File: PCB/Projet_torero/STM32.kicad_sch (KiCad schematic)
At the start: 35 parts, among them J201 Conn_02x07_Odd_Even, J202 Conn_02x08_Odd_Even, SW201 SW_Push, SW202 SW_Push, U201 STM32G431CBUx, Y201 Crystal_GND24_Small

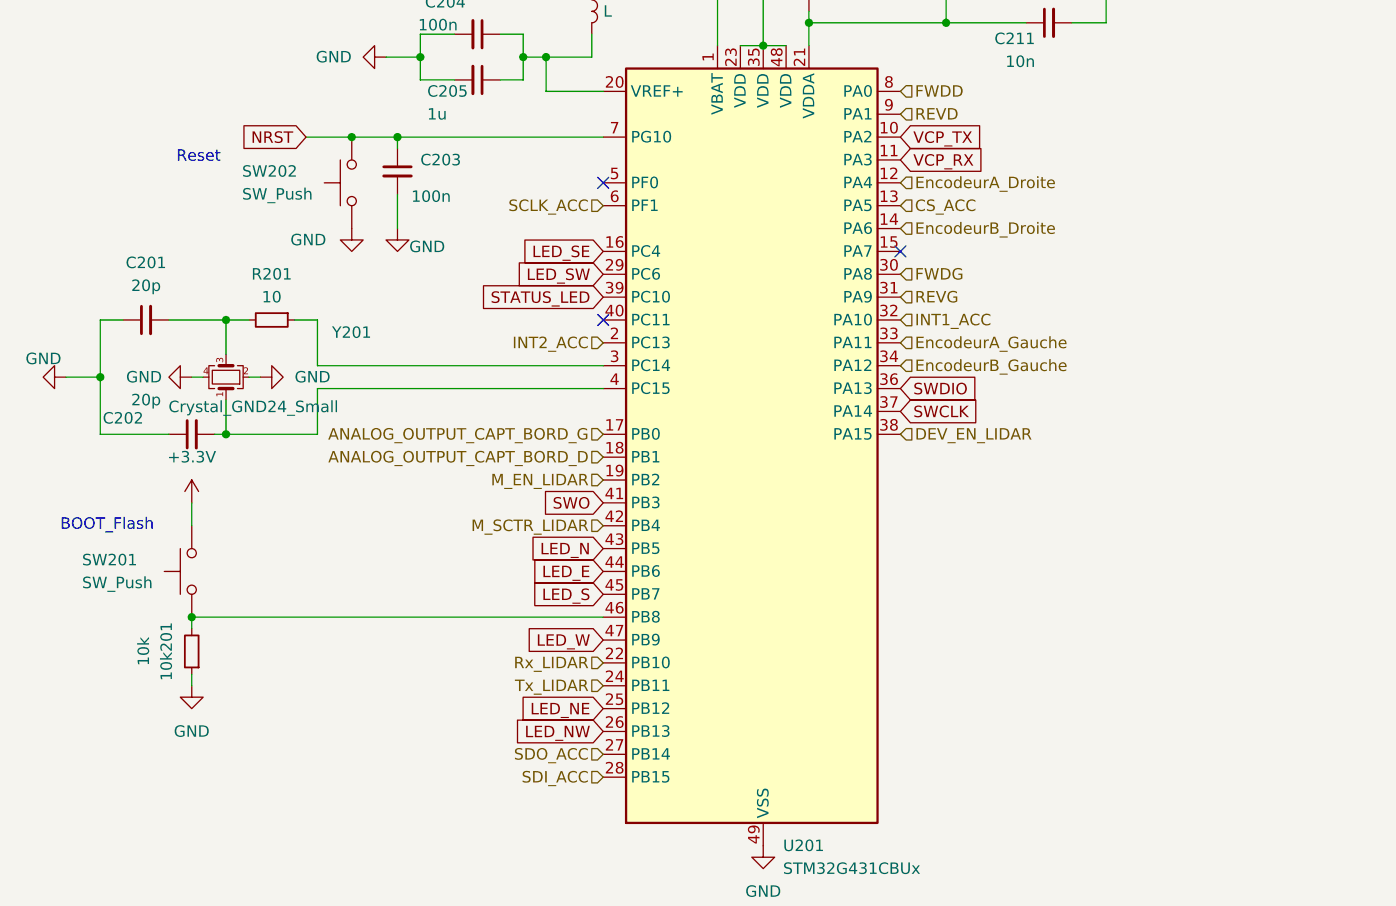
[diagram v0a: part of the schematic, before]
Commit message: maj pin STM
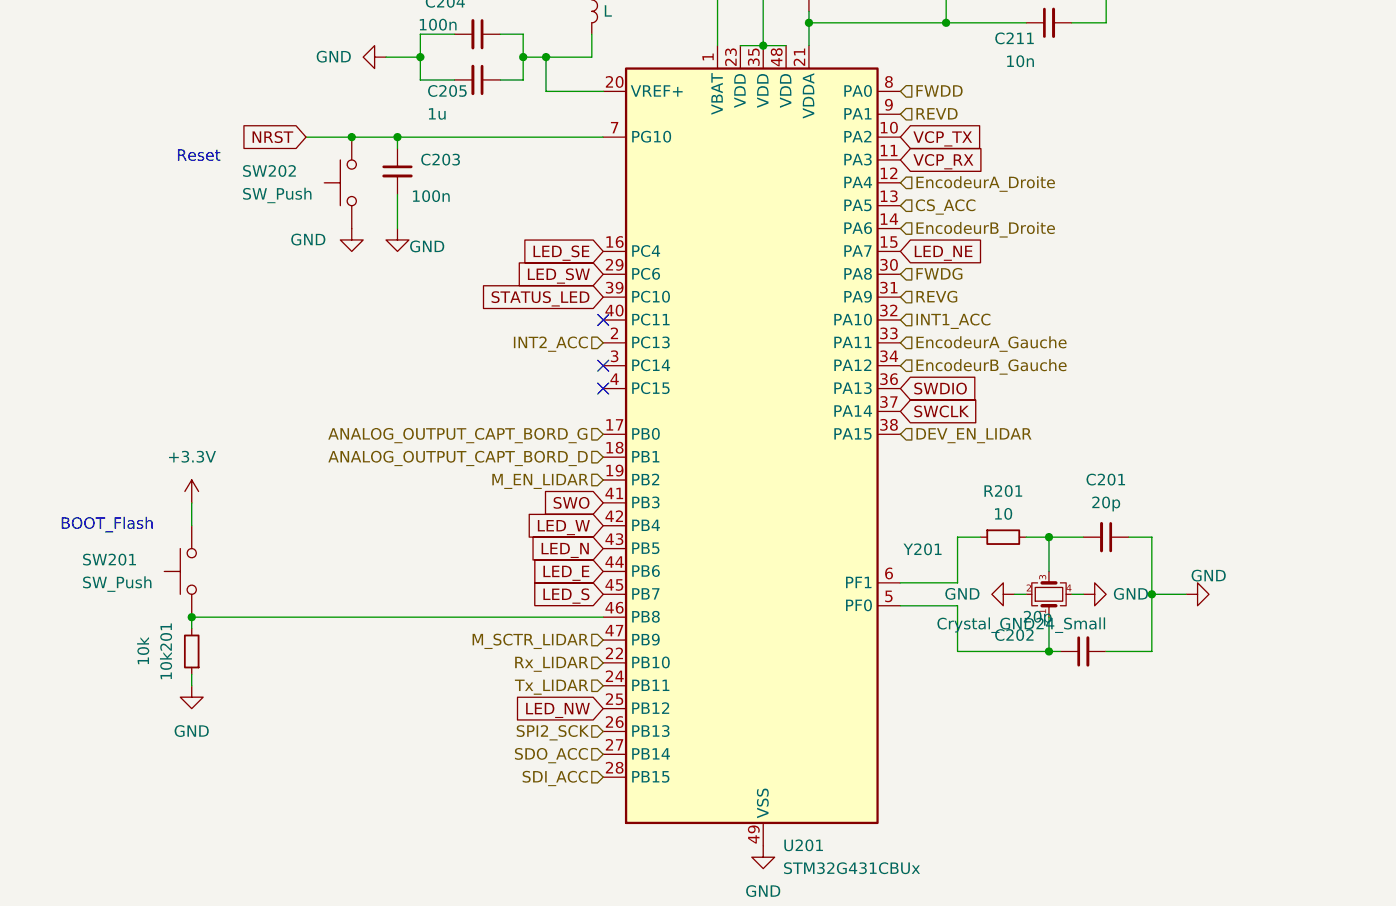
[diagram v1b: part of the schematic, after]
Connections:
- net SCLK_ACC is gone; now on an unnamed net: U201.6 (PF1)
- net GND: now also C202.2; no longer C202.1
- net LED_NE: now also U201.15 (PA7); no longer U201.25 (PB12)
- net LED_NW: now also U201.25 (PB12); no longer U201.26 (PB13)
- net LED_W: now also U201.42 (PB4); no longer U201.47 (PB9)
- net M_SCTR_LIDAR: now also U201.47 (PB9); no longer U201.42 (PB4)
- net at R201.1: no longer U201.3 (PC14)
- net at U201.5 (PF0): now also C202.1, Y201.1
- new net SPI2_SCK: U201.26 (PB13)
- now unconnected: U201.4 (PC15)
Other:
- moved on the sheet: C201, C202, R201, Y201
